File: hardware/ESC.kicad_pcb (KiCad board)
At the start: 4 copper layers, 52 x 25 mm, 85 parts, among them J1 +, J2 -, J3 +, J4 +, J5 +, J6 +, J7 Conn_01x03, J8 +, J9 +, Q1 AGM60P30AP, Q2 AGM60P30AP, Q3 AGM60P30AP, Q4 AGM60P30AP, Q5 AGM60P30AP, Q6 AGM60P30AP, Q7 AGM60P30A, U1 DRV8323RSRGZR, U2 STM32G431CBTx, Y1 X322516MLB4SI

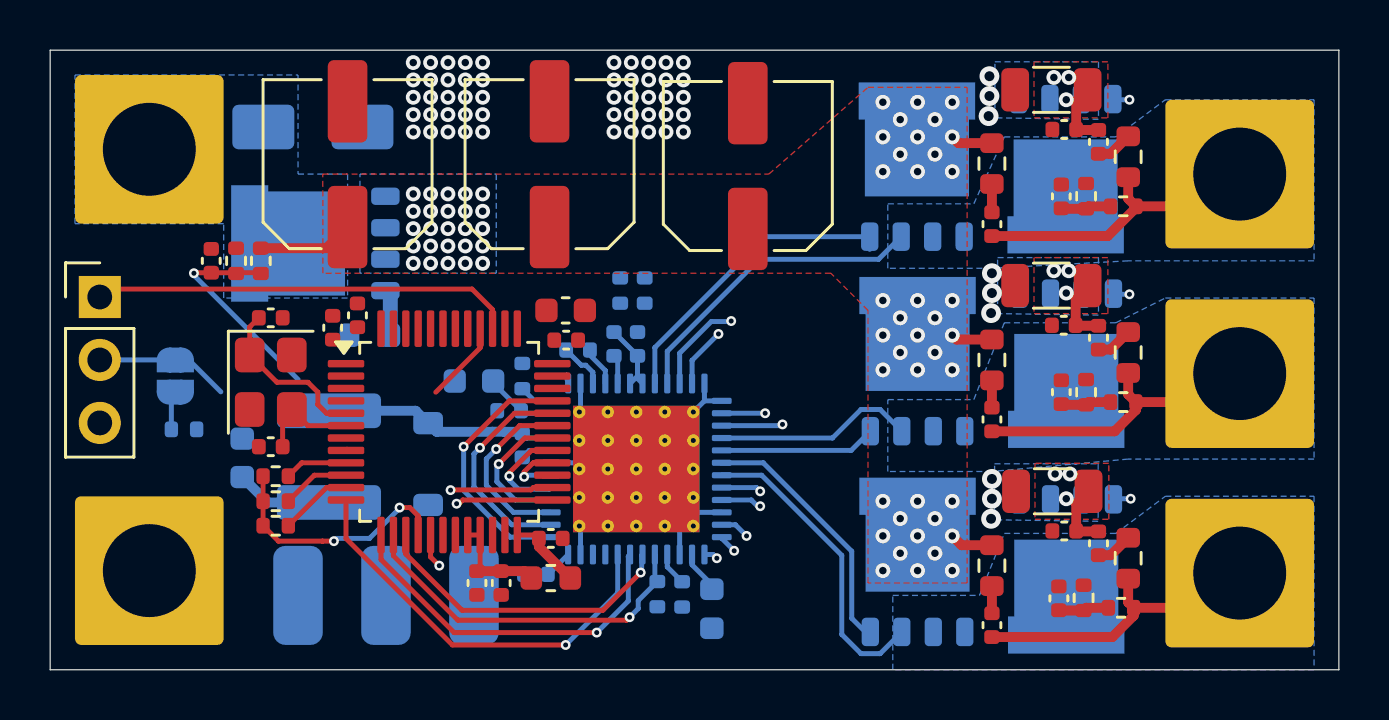
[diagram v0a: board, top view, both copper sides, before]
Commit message: finished pcb
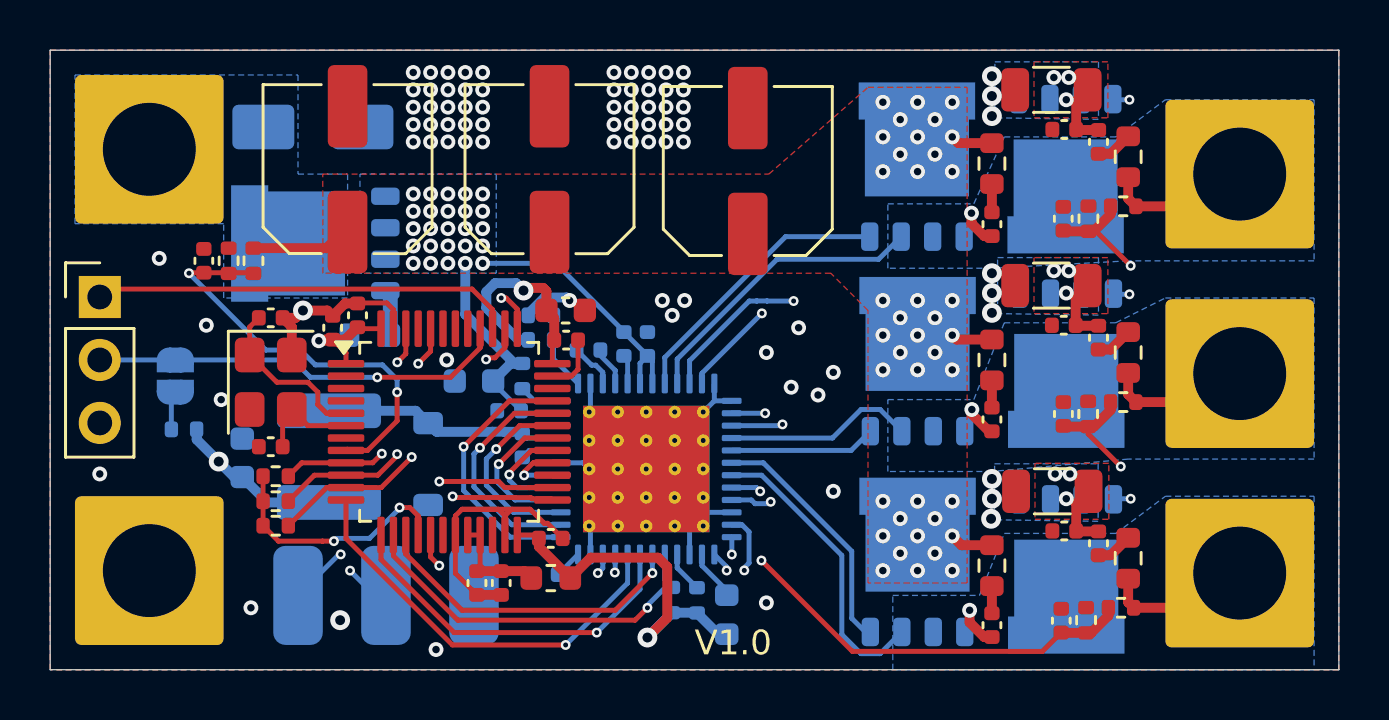
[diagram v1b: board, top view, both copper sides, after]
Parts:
- moved R12 4.31 mm to (157.8, 95.7), turned to 0 degrees
- moved R11 3.77 mm to (157.8, 96.7), turned to 180 degrees
- moved R19 0.91 mm to (179.9, 91.8)
- moved R23 0.91 mm to (179.8, 108.0)
- moved C25 0.91 mm to (178.8, 108.0)
- moved C23 0.90 mm to (178.9, 91.8)
- moved C22 0.88 mm to (178.9, 99.7)
- moved R17 0.88 mm to (179.9, 99.7)
- moved FB1 0.65 mm to (165.3, 107.8)
- moved R14 0.65 mm to (164.1, 107.2)
- moved R15 0.65 mm to (163.1, 107.2)
- moved C11 0.42 mm to (159.7, 97.1)
- moved C10 0.40 mm to (162.1, 96.9)
- moved C12 0.40 mm to (161.2, 96.9)
- moved C13 0.40 mm to (158.0, 106.2)
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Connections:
- U2 pad 44: unconnected-(U2-PB7-Pad44) -> /DRV_CAL
- U2 pad 46: unconnected-(U2-PB9-Pad46) -> /DRV_EN
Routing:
- net +3.3V: track 6.98 -> 46.9 mm, vias 0 -> 5
- net /BEMF_A: track 4.59 -> 42.7 mm, vias 0 -> 2
- net /BEMF_B: track 4.81 -> 41.5 mm, vias 0 -> 2
- net /BEMF_C: track 5.02 -> 38.4 mm, vias 0 -> 2
- net /DRV_EN: track 0.00 -> 25.4 mm, vias 0 -> 2
- net /DRV_CAL: track 0.00 -> 23.7 mm, vias 0 -> 2
- net GND: track 17.5 -> 36.5 mm, vias 59 -> 78
- net /SWDIO: track 0.00 -> 17.3 mm, vias 0 -> 2
- net /SWCLK: track 0.00 -> 14.5 mm, vias 0 -> 2
- net VBUS: track 15.5 -> 29.3 mm
- net /IN_ADC: track 8.78 -> 17.0 mm, vias 1 -> 2
- net /DIR: track 8.72 -> 16.9 mm, vias 0 -> 1
- net /MOTOR_B: track 20.6 -> 15.0 mm, vias 0 -> 1
- net /MOTOR_A: track 31.2 -> 25.8 mm, vias 0 -> 1
- net /MOTOR_C: track 25.0 -> 19.8 mm, vias 0 -> 1
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- added copper zone on In2.Cu, net +3.3V
- added copper zone on B.Cu, net GND
- added copper zone on F.Cu, net GND
- added copper zone on In1.Cu, net GND
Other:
- board text added: "CCW"
- board text added: "CW"
- board text added: "V1.0"
